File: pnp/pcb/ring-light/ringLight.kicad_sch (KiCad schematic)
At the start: 21 parts, among them J1 Connector Top, J2 Connector Bot

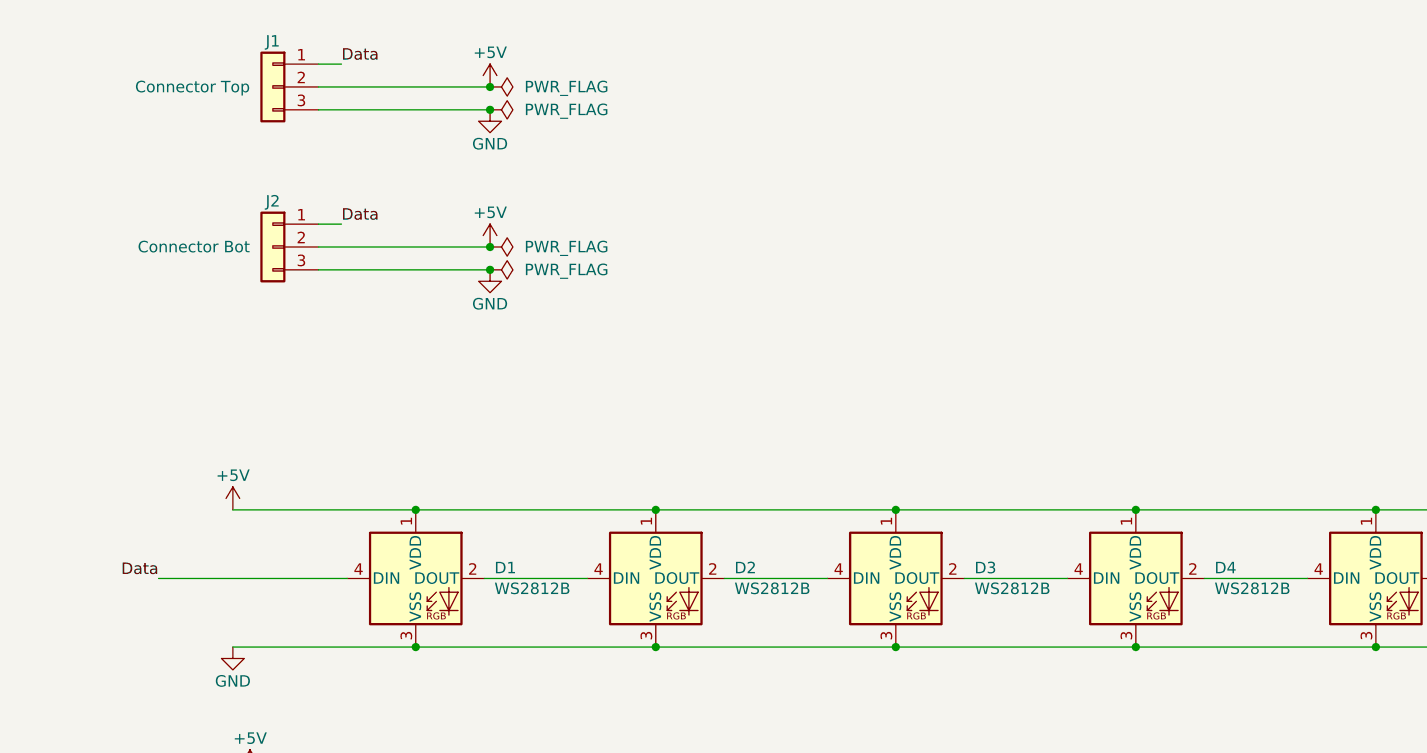
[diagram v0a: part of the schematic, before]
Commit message: reverts ring light to original design with level shifters
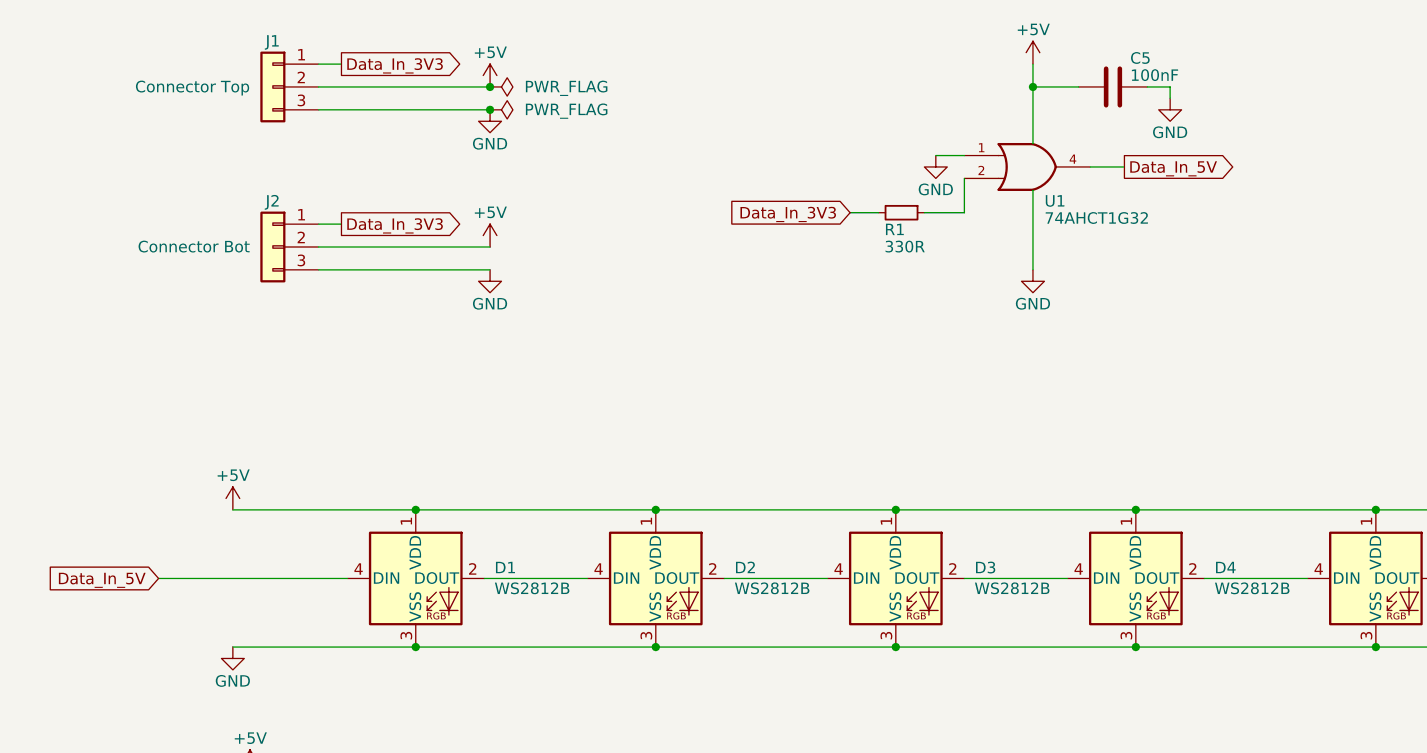
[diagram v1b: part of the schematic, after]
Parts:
- added C5: 100nF, Capacitor_SMD:C_0805_2012Metric, symbol Device:C
- added R1: 330R, Resistor_SMD:R_0805_2012Metric, symbol Device:R_Small
- added U1: 74AHCT1G32, Package_TO_SOT_SMD:SOT-353_SC-70-5, symbol 74xGxx:74AHCT1G32
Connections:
- net +5V: now also C5.1, U1.5 (VCC)
- net GND: now also C5.2, U1.1, U1.3 (GND)
- net Data renamed Data_In_3V3
- net Data_In_3V3: now also R1.2; no longer D1.4 (DIN)
- new net: R1.1, U1.2
- new net Data_In_5V: D1.4 (DIN), U1.4
